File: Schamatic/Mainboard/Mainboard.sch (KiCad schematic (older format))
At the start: 101 parts, among them J1 BAT+, J10 BAT-, J11 PLUG+, J12 PLUG-, J13 MOUNT, J14 MOUNT, J15 MOUNT, J16 MOUNT, J2 M+1, J3 USART, J4 3.3V, J5 CONN_02X04, J6 JTAG, J7 M+2, J8 M-1, J9 M-2, Q1 p-MOSFET, SW1 B3U-1000P, SW2 B3U-1000P, SW3 B3U-1000P, SW4 B3U-1000P, SW5 B3U-1000P, U1 ACS781, U2 ADP2303ARDZ-3.3, U3 cc3220, U4 DEA202450BT-3201B2, U5 MX25R3235F, U6 LSM9DS1, U7 LTC2954, U8 LTC2876, Y1 32.768kHz, Y2 40Mhz

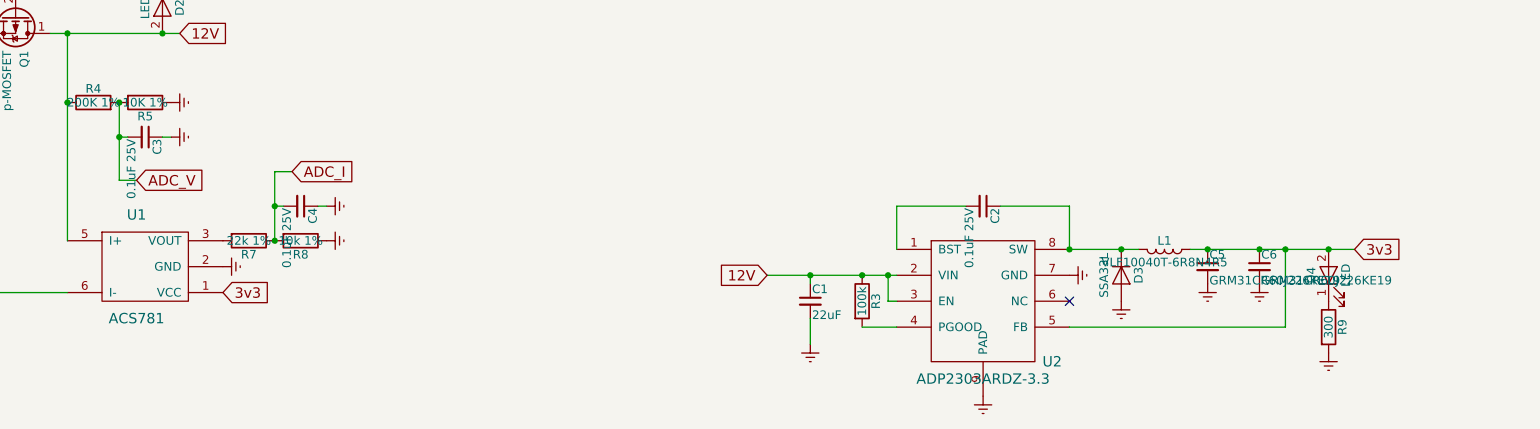
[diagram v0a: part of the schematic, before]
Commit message: minor corrections
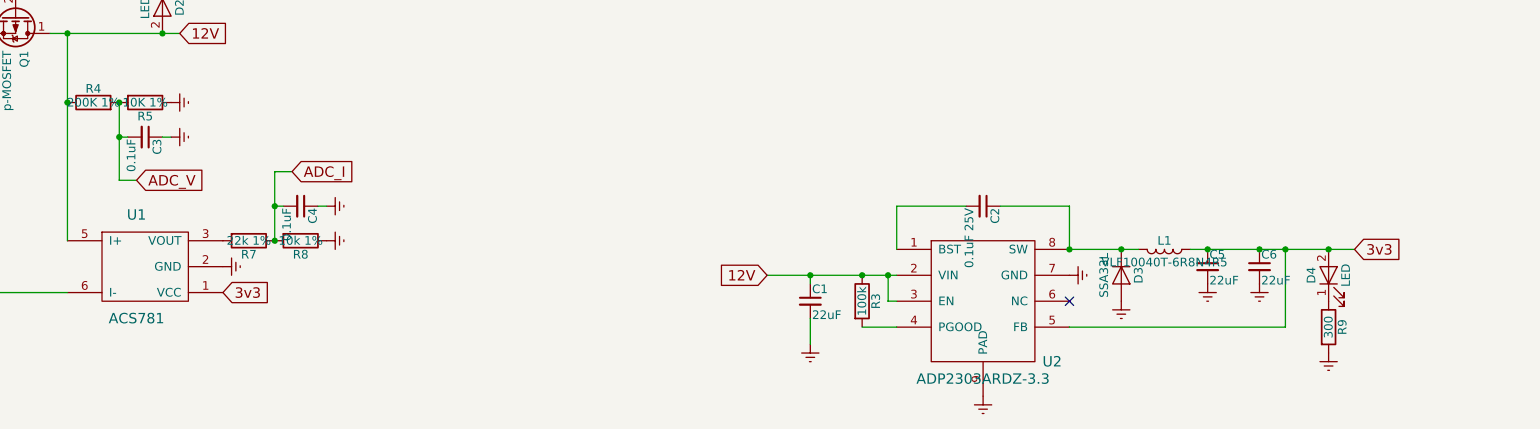
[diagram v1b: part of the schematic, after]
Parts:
- C3, C4: value 0.1uF 25V -> 0.1uF
- C5, C6: value GRM31CR60J226KE19 -> 22uF
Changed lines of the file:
@@
 P 9050 9850
 F 0 "C5" H 9060 9920 50  0000 L CNN
-F 1 "GRM31CR60J226KE19" H 9060 9770 50  0000 L CNN
+F 1 "22uF" H 9060 9770 50  0000 L CNN
 F 2 "Capacitors_SMD:C_1206" H 9050 9850 50  0001 C CNN
 F 3 "" H 9050 9850 50  0001 C CNN
@@
 P 9350 9850
 F 0 "C6" H 9360 9920 50  0000 L CNN
-F 1 "GRM31CR60J226KE19" H 9360 9770 50  0000 L CNN
+F 1 "22uF" H 9360 9770 50  0000 L CNN
 F 2 "Capacitors_SMD:C_1206" H 9350 9850 50  0001 C CNN
 F 3 "" H 9350 9850 50  0001 C CNN
@@
 P 2900 9100
 F 0 "C3" H 2910 9170 50  0000 L CNN
-F 1 "0.1uF 25V" H 2910 9020 50  0000 L CNN
+F 1 "0.1uF" H 2910 9020 50  0000 L CNN
 F 2 "Capacitors_SMD:C_0603" H 2900 9100 50  0001 C CNN
 F 3 "" H 2900 9100 50  0001 C CNN
@@
 P 3800 9500
 F 0 "C4" H 3810 9570 50  0000 L CNN
-F 1 "0.1uF 25V" H 3810 9420 50  0000 L CNN
+F 1 "0.1uF" H 3810 9420 50  0000 L CNN
 F 2 "Capacitors_SMD:C_0603" H 3800 9500 50  0001 C CNN
 F 3 "" H 3800 9500 50  0001 C CNN
